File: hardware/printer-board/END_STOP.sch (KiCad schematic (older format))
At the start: 27 parts, among them J15 X_MIN, J16 X_MAX, J17 Y_MIN, J18 Y_MAX, J19 Z_MIN, J20 Z_MAX, J45 END_SWITCH_DEBUG, J48 HOTEND_PROBE

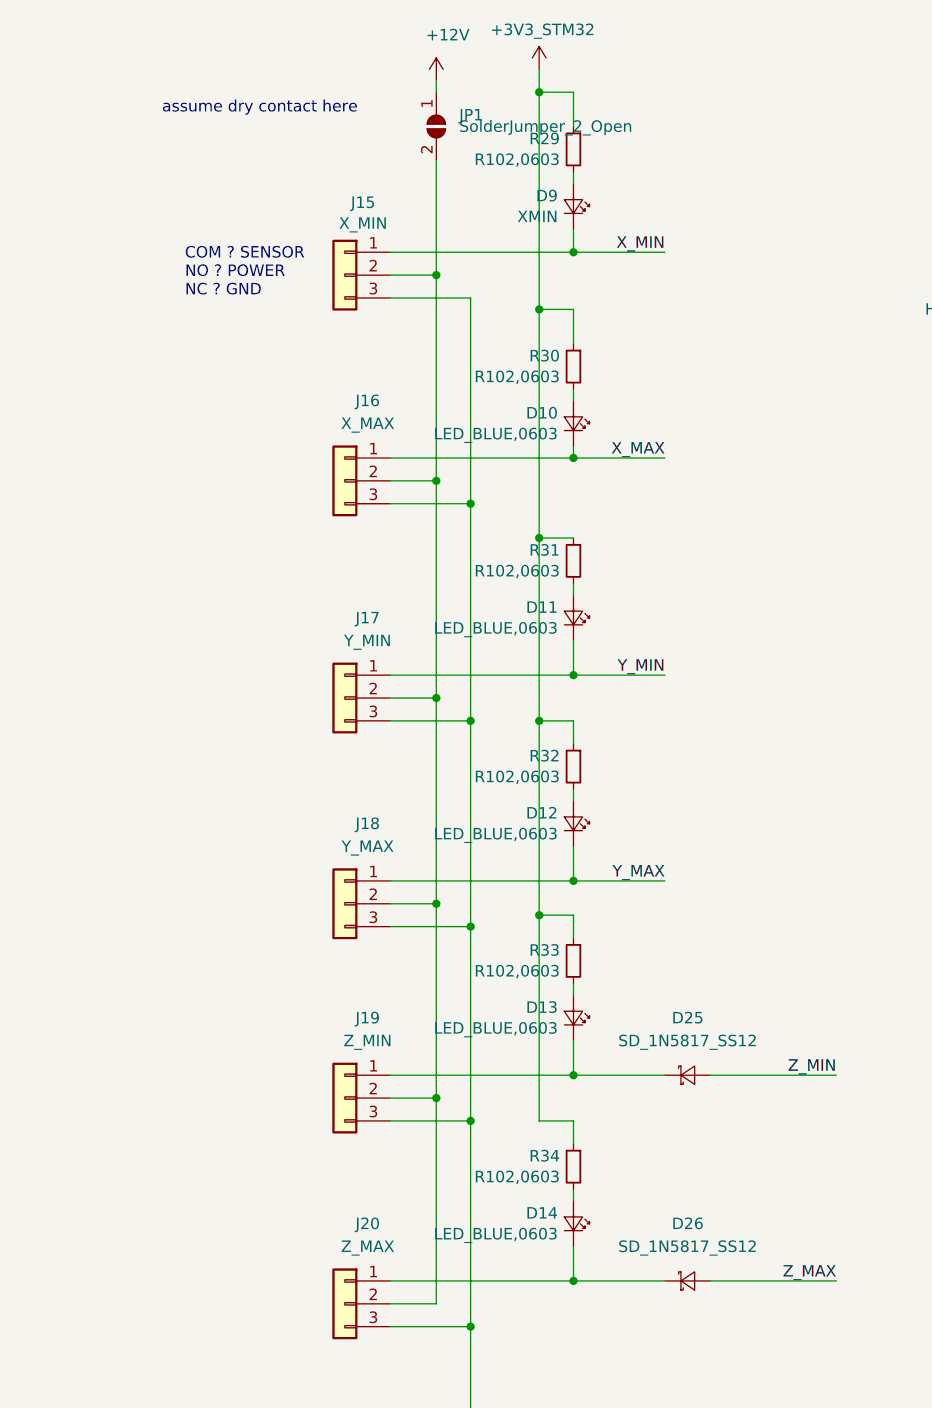
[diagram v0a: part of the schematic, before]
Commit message: update ROUTING,
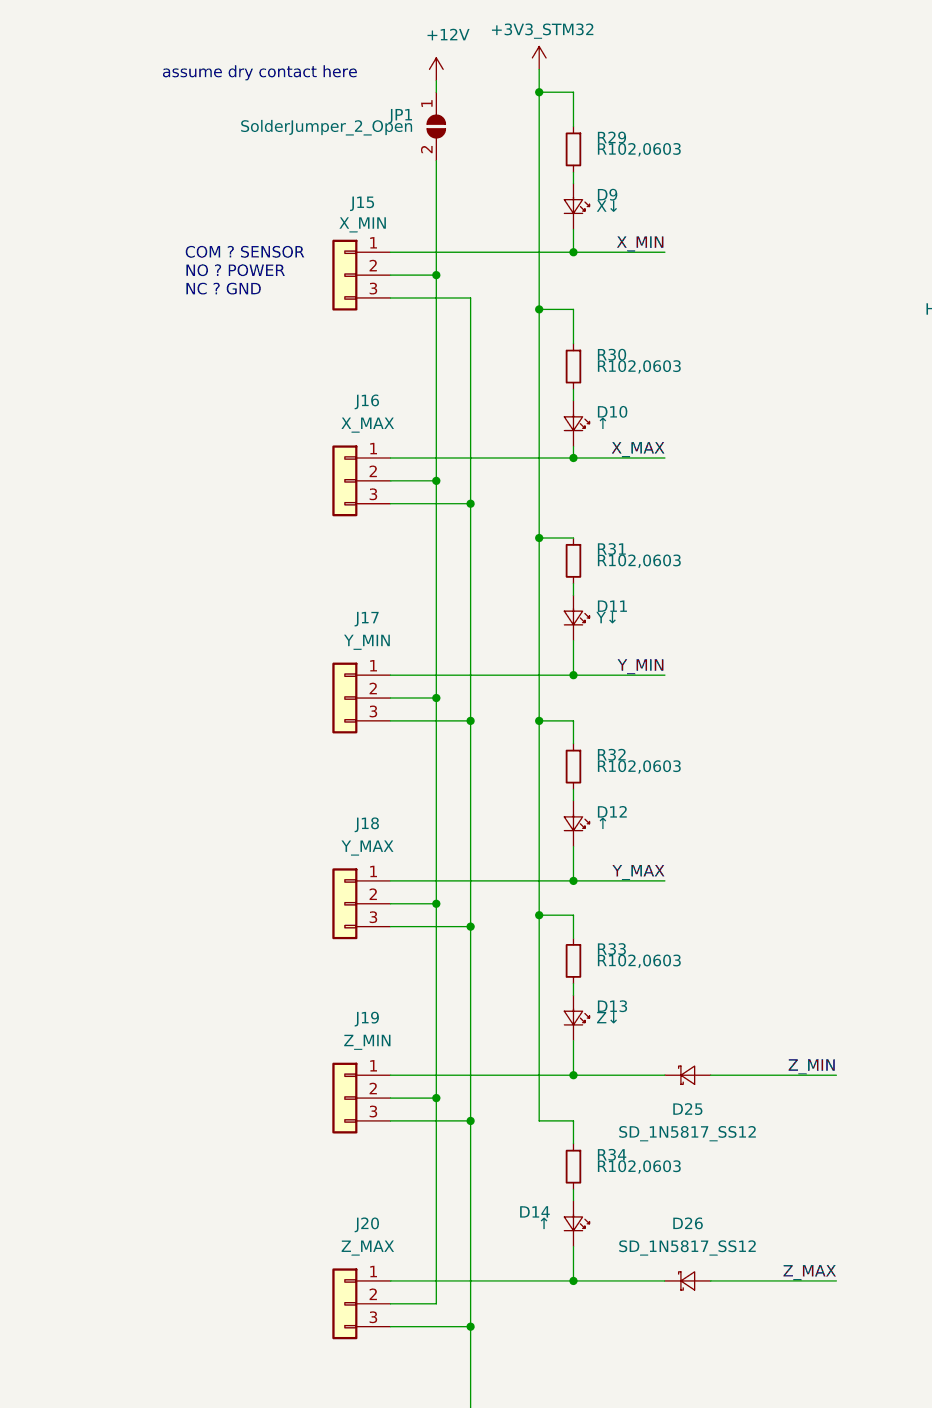
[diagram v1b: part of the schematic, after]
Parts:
- D10, D12, D14: value LED_BLUE,0603 -> ↑
- D11: value LED_BLUE,0603 -> Y↓
- D13: value LED_BLUE,0603 -> Z↓
- D9: value XMIN -> X↓
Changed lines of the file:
@@
 U 1 1 5CC31819
 P 4250 1450
-F 0 "R29" H 4309 1496 50  0000 L CNN
-F 1 "R102,0603" H 4309 1405 50  0000 L CNN
+F 0 "R29" H 4150 1500 50  0000 R CNN
+F 1 "R102,0603" H 4150 1450 50  0000 R CNN
 F 2 "Resistor_SMD:R_0603_1608Metric_Pad1.05x0.95mm_HandSolder" H 4250 1450 50  0001 C CNN
 F 3 "~" H 4250 1450 50  0001 C CNN
@@
 U 1 1 5CC31941
 P 4250 1700
-F 0 "D9" V 4296 1632 50  0000 R CNN
-F 1 "XMIN" V 4205 1632 50  0000 R CNN
+F 0 "D9" V 4300 1800 50  0000 L CNN
+F 1 "X↓" V 4250 1800 50  0000 L CNN
 F 2 "LED_SMD:LED_0603_1608Metric_Pad1.05x0.95mm_HandSolder" V 4250 1700 50  0001 C CNN
 F 3 "" V 4250 1700 50  0001 C CNN
@@
 U 1 1 5CC33066
 P 4250 2400
-F 0 "R30" H 4309 2446 50  0000 L CNN
-F 1 "R102,0603" H 4309 2355 50  0000 L CNN
+F 0 "R30" H 4150 2450 50  0000 R CNN
+F 1 "R102,0603" H 4150 2400 50  0000 R CNN
 F 2 "Resistor_SMD:R_0603_1608Metric_Pad1.05x0.95mm_HandSolder" H 4250 2400 50  0001 C CNN
 F 3 "~" H 4250 2400 50  0001 C CNN
@@
 U 1 1 5CC3306C
 P 4250 2650
-F 0 "D10" V 4296 2582 50  0000 R CNN
-F 1 "LED_BLUE,0603" V 4205 2582 50  0000 R CNN
+F 0 "D10" V 4300 2750 50  0000 L CNN
+F 1 "↑" V 4250 2750 50  0000 L CNN
 F 2 "LED_SMD:LED_0603_1608Metric_Pad1.05x0.95mm_HandSolder" V 4250 2650 50  0001 C CNN
 F 3 "" V 4250 2650 50  0001 C CNN
@@
 U 1 1 5CC3434E
 P 4250 3250
-F 0 "R31" H 4309 3296 50  0000 L CNN
-F 1 "R102,0603" H 4309 3205 50  0000 L CNN
+F 0 "R31" H 4150 3300 50  0000 R CNN
+F 1 "R102,0603" H 4150 3250 50  0000 R CNN
 F 2 "Resistor_SMD:R_0603_1608Metric_Pad1.05x0.95mm_HandSolder" H 4250 3250 50  0001 C CNN
 F 3 "~" H 4250 3250 50  0001 C CNN
@@
 U 1 1 5CC34354
 P 4250 3500
-F 0 "D11" V 4296 3432 50  0000 R CNN
-F 1 "LED_BLUE,0603" V 4205 3432 50  0000 R CNN
+F 0 "D11" V 4300 3600 50  0000 L CNN
+F 1 "Y↓" V 4250 3600 50  0000 L CNN
 F 2 "LED_SMD:LED_0603_1608Metric_Pad1.05x0.95mm_HandSolder" V 4250 3500 50  0001 C CNN
 F 3 "" V 4250 3500 50  0001 C CNN
@@
 U 1 1 5CC34FAC
 P 4250 4150
-F 0 "R32" H 4309 4196 50  0000 L CNN
-F 1 "R102,0603" H 4309 4105 50  0000 L CNN
+F 0 "R32" H 4150 4200 50  0000 R CNN
+F 1 "R102,0603" H 4150 4150 50  0000 R CNN
 F 2 "Resistor_SMD:R_0603_1608Metric_Pad1.05x0.95mm_HandSolder" H 4250 4150 50  0001 C CNN
 F 3 "~" H 4250 4150 50  0001 C CNN
@@
 U 1 1 5CC34FB2
 P 4250 4400
-F 0 "D12" V 4296 4332 50  0000 R CNN
-F 1 "LED_BLUE,0603" V 4205 4332 50  0000 R CNN
+F 0 "D12" V 4300 4500 50  0000 L CNN
+F 1 "↑" V 4250 4500 50  0000 L CNN
 F 2 "LED_SMD:LED_0603_1608Metric_Pad1.05x0.95mm_HandSolder" V 4250 4400 50  0001 C CNN
 F 3 "" V 4250 4400 50  0001 C CNN
@@
 U 1 1 5CC35E90
 P 4250 5000
-F 0 "R33" H 4309 5046 50  0000 L CNN
-F 1 "R102,0603" H 4309 4955 50  0000 L CNN
+F 0 "R33" H 4150 5050 50  0000 R CNN
+F 1 "R102,0603" H 4150 5000 50  0000 R CNN
 F 2 "Resistor_SMD:R_0603_1608Metric_Pad1.05x0.95mm_HandSolder" H 4250 5000 50  0001 C CNN
 F 3 "~" H 4250 5000 50  0001 C CNN
@@
 U 1 1 5CC35E96
 P 4250 5250
-F 0 "D13" V 4296 5182 50  0000 R CNN
-F 1 "LED_BLUE,0603" V 4205 5182 50  0000 R CNN
+F 0 "D13" V 4300 5350 50  0000 L CNN
+F 1 "Z↓" V 4250 5350 50  0000 L CNN
 F 2 "LED_SMD:LED_0603_1608Metric_Pad1.05x0.95mm_HandSolder" V 4250 5250 50  0001 C CNN
 F 3 "" V 4250 5250 50  0001 C CNN
@@
 U 1 1 5CC36FE8
 P 4250 5900
-F 0 "R34" H 4309 5946 50  0000 L CNN
-F 1 "R102,0603" H 4309 5855 50  0000 L CNN
+F 0 "R34" H 4150 5950 50  0000 R CNN
+F 1 "R102,0603" H 4150 5900 50  0000 R CNN
 F 2 "Resistor_SMD:R_0603_1608Metric_Pad1.05x0.95mm_HandSolder" H 4250 5900 50  0001 C CNN
 F 3 "~" H 4250 5900 50  0001 C CNN
@@
 U 1 1 5CC36FEE
 P 4250 6150
-F 0 "D14" V 4296 6082 50  0000 R CNN
-F 1 "LED_BLUE,0603" V 4205 6082 50  0000 R CNN
+F 0 "D14" V 4300 6050 50  0000 R CNN
+F 1 "↑" V 4250 6050 50  0000 R CNN
 F 2 "LED_SMD:LED_0603_1608Metric_Pad1.05x0.95mm_HandSolder" V 4250 6150 50  0001 C CNN
 F 3 "" V 4250 6150 50  0001 C CNN
@@
 U 1 1 5CD6EA2D
 P 3650 1350
-F 0 "JP1" V 3600 1450 50  0000 L CNN
-F 1 "SolderJumper_2_Open" V 3650 1450 50  0000 L CNN
+F 0 "JP1" V 3600 1250 50  0000 R CNN
+F 1 "SolderJumper_2_Open" V 3650 1250 50  0000 R CNN
 F 2 "Jumper:SolderJumper-2_P1.3mm_Open_RoundedPad1.0x1.5mm" H 3650 1350 50  0001 C CNN
 F 3 "~" H 3650 1350 50  0001 C CNN
@@
 Wire Wire Line
 	6750 1250 6750 1300
-Text Notes 2450 1300 0    50   ~ 0
+Text Notes 2450 1150 0    50   ~ 0
 assume dry contact here
 Wire Notes Line
@@
 U 1 1 5CD8DF8F
 P 4750 5500
-F 0 "D25" H 4750 5750 50  0000 C CNN
-F 1 "SD_1N5817_SS12" H 4750 5650 50  0000 C CNN
+F 0 "D25" H 4750 5350 50  0000 C CNN
+F 1 "SD_1N5817_SS12" H 4750 5250 50  0000 C CNN
 F 2 "w_smd_diode:do214ac" V 4750 5500 50  0001 C CNN
 F 3 "~" V 4750 5500 50  0001 C CNN
